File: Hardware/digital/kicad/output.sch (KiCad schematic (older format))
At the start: 11 parts, among them J1 CONN-SMA-5-1814400-1, J2 Micro_SD, Q1 NTR4501N, U3 RFM69CW, U4 SIM800L, U5 huzzah

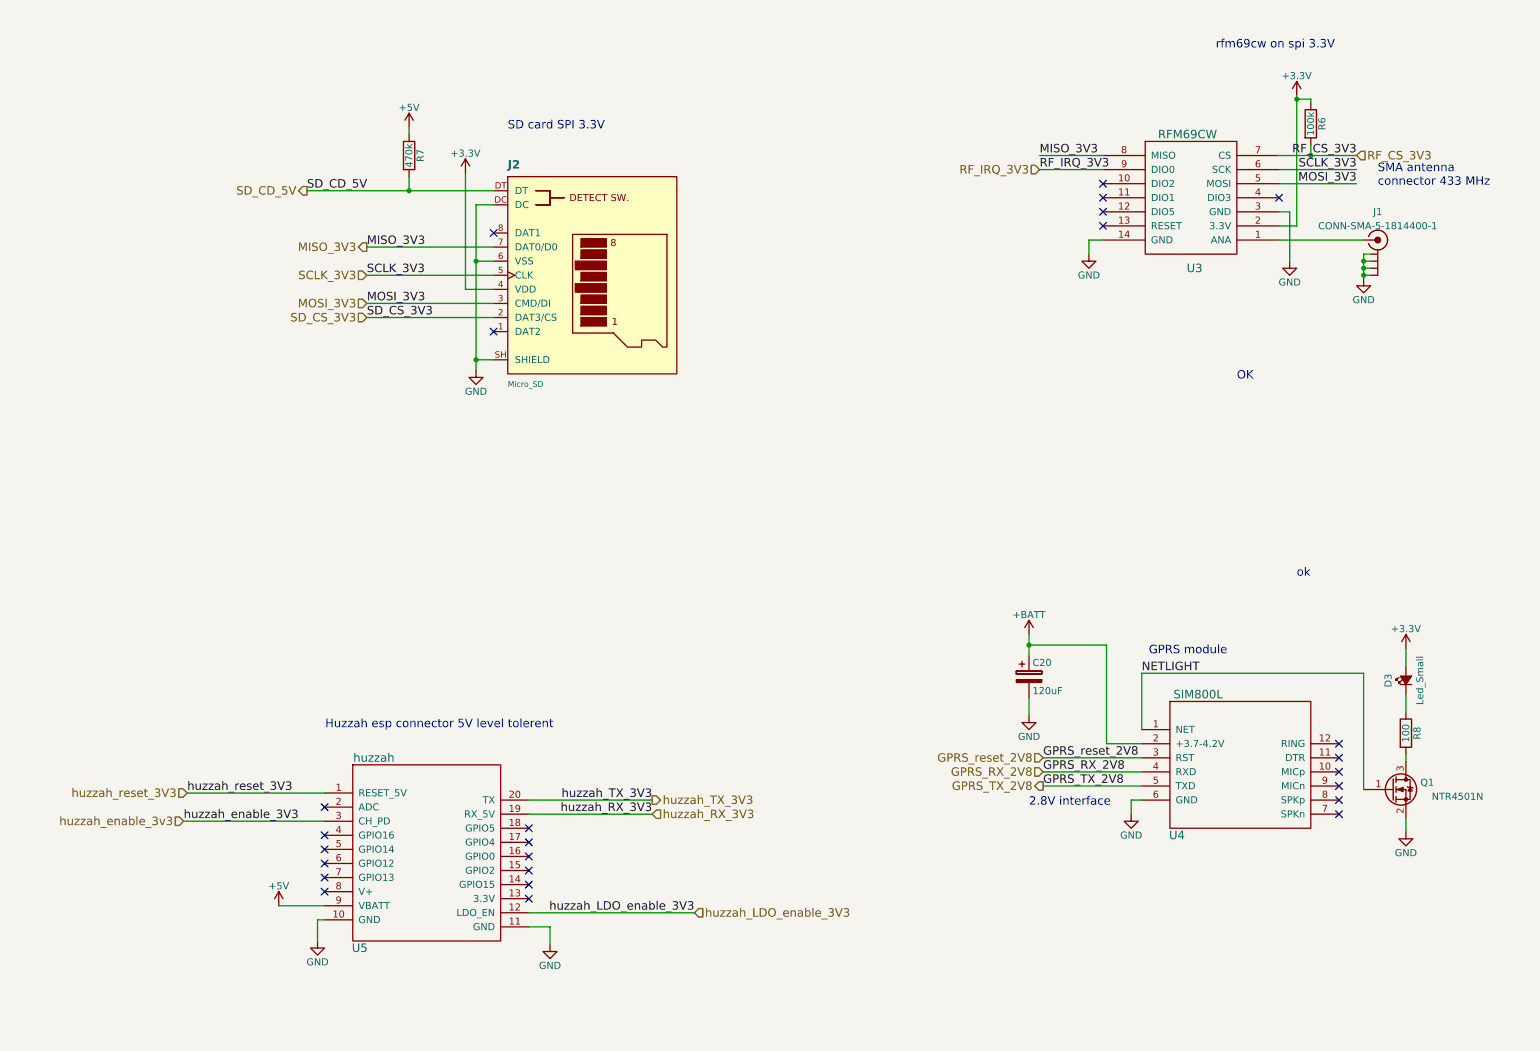
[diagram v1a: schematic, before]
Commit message: move to digital 1.1.1
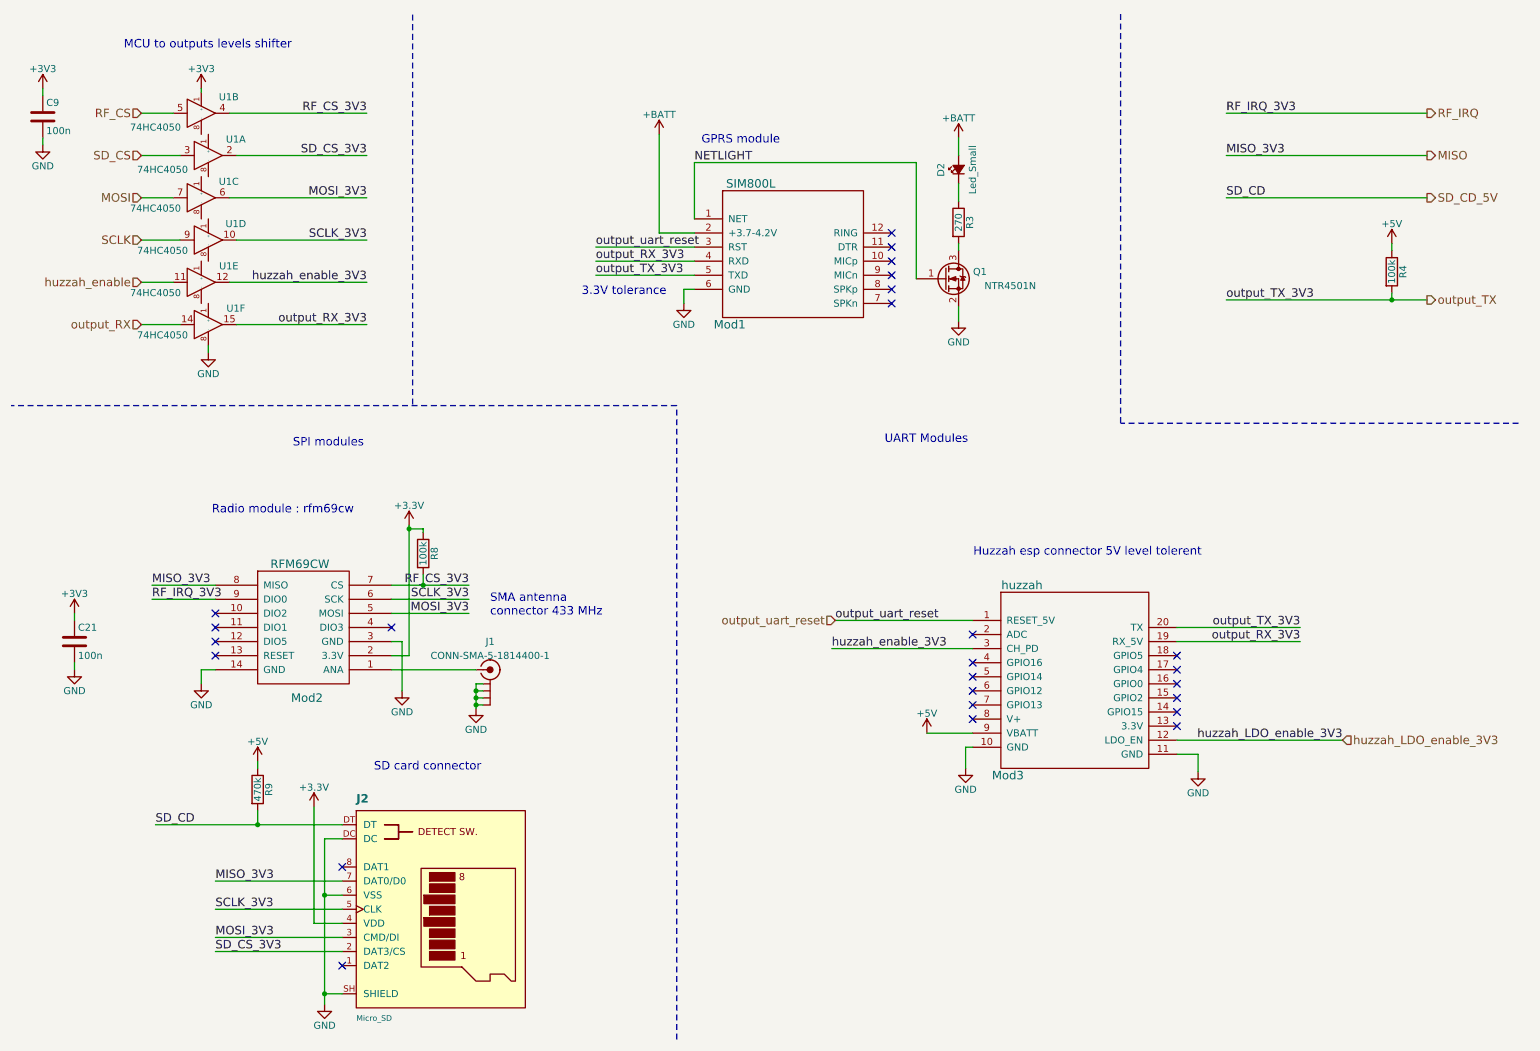
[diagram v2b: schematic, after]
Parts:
- removed C20: 120uF, Capacitors_ThroughHole:C_Radial_D6.3_L11.2_P2.5, symbol CP
- added C21, C9: 100n, Capacitors_ThroughHole:C_Rect_L7_W2.5_P5, symbol C
- added R4: 100k, Resistors_ThroughHole:Resistor_Horizontal_RM10mm, symbol R
- added U1: 74HC4050, Housings_SOIC:SOIC-16_3.9x9.9mm_Pitch1.27mm, symbol 74HC4050
- R3: renamed from R8; value 100 -> 270; footprint Discret:R3-LARGE_PADS -> Resistors_ThroughHole:Resistor_Horizontal_RM10mm
- R8: renamed from R6; footprint Discret:R3-LARGE_PADS -> Resistors_ThroughHole:Resistor_Horizontal_RM10mm
- R9: renamed from R7; footprint Discret:R3-LARGE_PADS -> Resistors_ThroughHole:Resistor_Horizontal_RM10mm
- renumbered D3 to D2, U4 to Mod1, U3 to Mod2, U5 to Mod3
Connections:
- net huzzah_RX_3V3 is gone; now on net output_RX_3V3: Mod3.19 (RX_5V)
- net huzzah_TX_3V3 is gone; now on net output_TX: Mod3.20 (TX)
- net huzzah_reset_3V3 is gone; now on net output_uart_reset: Mod3.1 (RESET_5V)
- net +3V3: now also C21.1, C9.1, U1.1 (+); no longer D2.2 (A)
- net +5V: now also R4.1
- net +BATT: now also D2.2 (A)
- net GND: now also C21.2, C9.2, U1.8 (-)
- net MOSI_3V3: now also U1.6
- net RF_CS_3V3: now also U1.4
- net SCLK_3V3: now also U1.10
- net SD_CS_3V3: now also U1.2
- net GPRS_RX_2V8 renamed output_RX_3V3
- net output_RX_3V3: now also U1.15
- net GPRS_TX_2V8 renamed output_TX
- net output_TX: now also R4.2
- net GPRS_reset_2V8 renamed output_uart_reset
- net MISO_3V3 renamed MISO
- net RF_IRQ_3V3 renamed RF_IRQ
- net huzzah_enable_3v3 renamed huzzah_enable_3V3
- net huzzah_enable_3V3: now also U1.12
- new net MOSI: U1.7
- new net RF_CS: U1.5
- new net SCLK: U1.9
- new net SD_CS: U1.3
- new net huzzah_enable: U1.11
- new net output_RX: U1.14
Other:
- note added: "3.3V tolerance"
- note added: "MCU to outputs levels shifter"
- note added: "Radio module : rfm69cw"
- note added: "SD card connector"
- note added: "SPI modules"
- note added: "UART Modules\n"
- note removed: "2.8V interface"
- note removed: "OK"
- note removed: "SD card SPI 3.3V"
- note removed: "ok"
- note removed: "rfm69cw on spi 3.3V"
- moved on the sheet: D2, J1, J2, Mod1, Mod2, Mod3, Q1, R3, R8, R9
